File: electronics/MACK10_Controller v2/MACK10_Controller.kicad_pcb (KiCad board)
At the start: 2 copper layers, 57.6 x 67.3 mm, 55 parts, among them J2 Motor, J3 J_Expansion, J4 I/O, J5 Sensor IDC, J6 Interface IDC, J7 Fan, J8 E_STOP, J9 24V IN, Q1 SS8550, U1 TMC2208, U2 HX711, U3 XIAO-C6, U4 INA226, U5 PCF8575, U6 MINI360

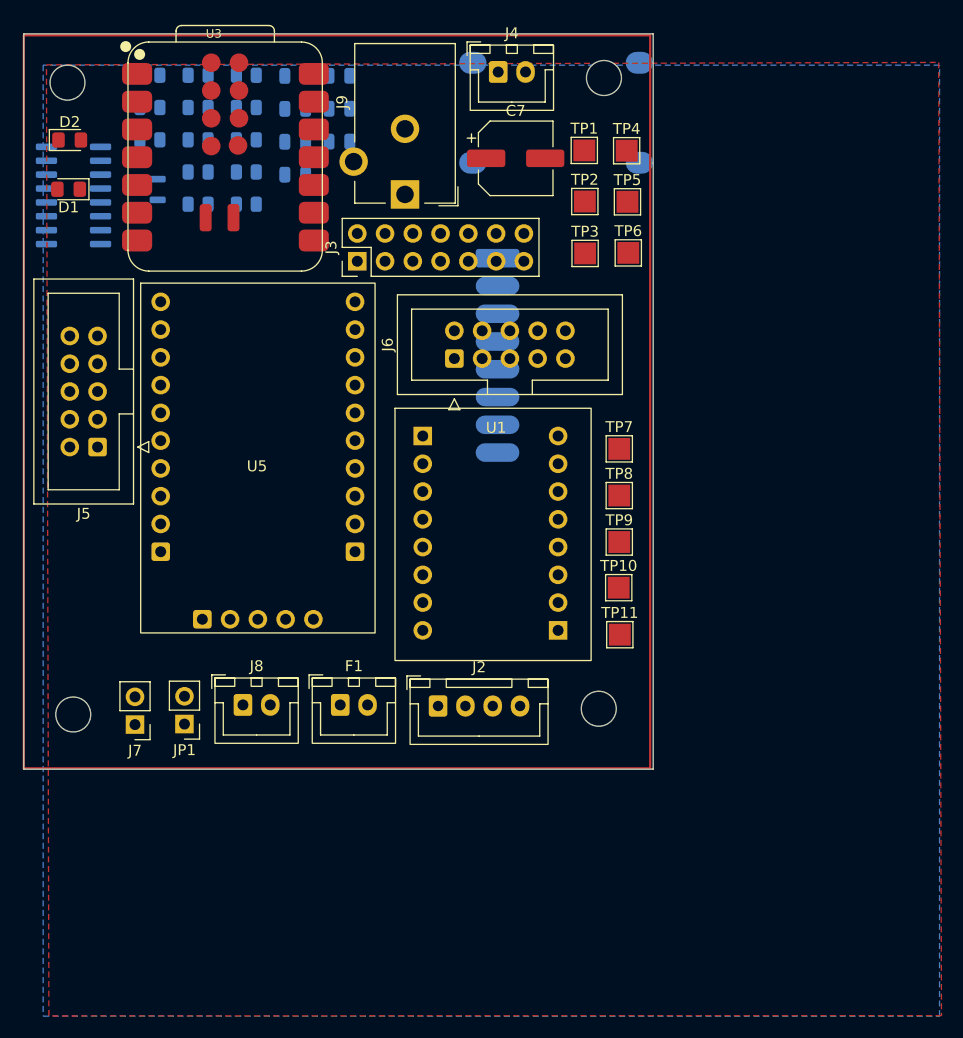
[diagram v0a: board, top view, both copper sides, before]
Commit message: PCB Layout Finalization
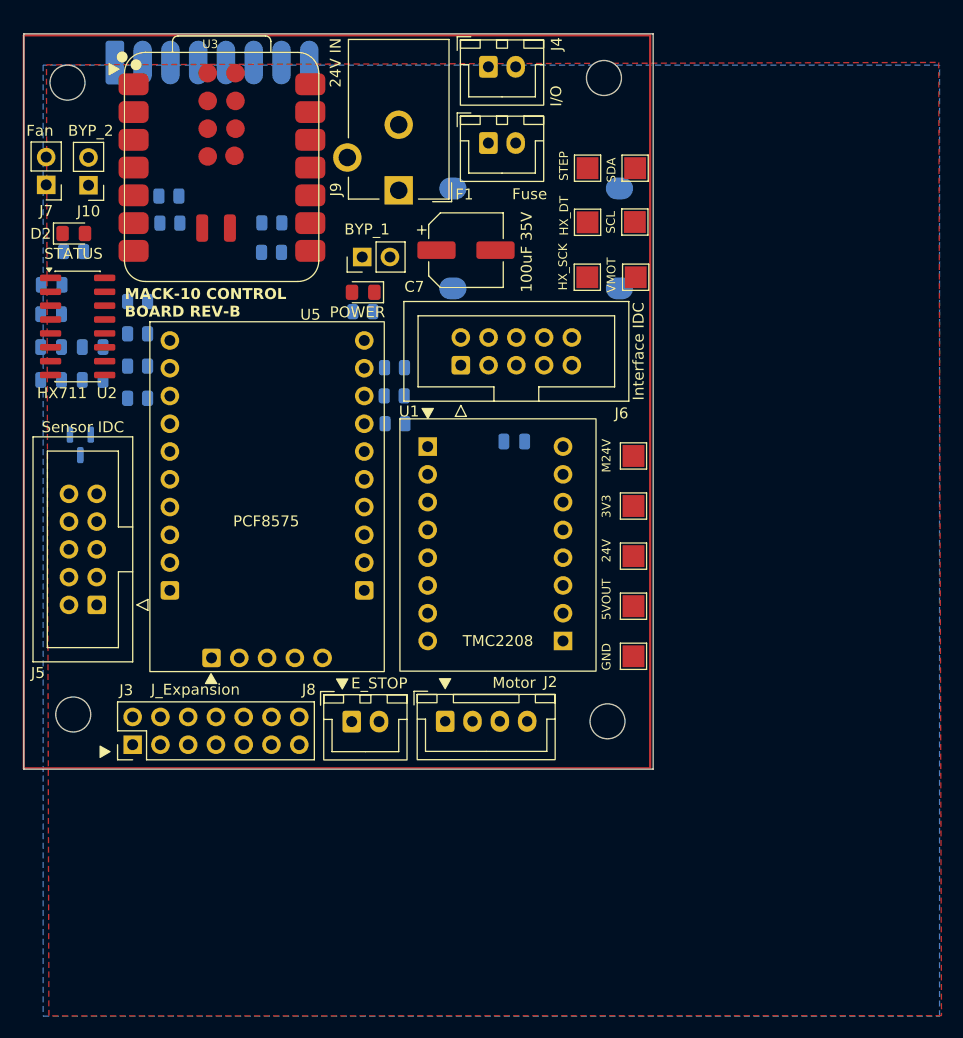
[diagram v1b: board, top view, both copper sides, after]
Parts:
- added J10: BYP_2, Connector_PinHeader_2.54mm:PinHeader_1x02_P2.54mm_Vertical, F.Cu at (23.1, 31.0)
- D2: value SMD_STATUS -> STATUS
- F1: value 2A Fuse -> Fuse
- JP1: value FUSE_BYPASS -> BYP_1
- U2: moved to F.Cu
- moved F1 53.2 mm to (59.7, 27.1)
- moved J7 50.0 mm to (19.3, 30.9)
- moved J3 48.8 mm to (27.2, 82.2)
- moved JP1 45.7 mm to (48.2, 37.5), turned to 90 degrees
- moved C5 37.1 mm to (62.1, 54.4)
- moved R8 31.6 mm to (51.2, 52.8)
- moved C6 31.4 mm to (23.5, 45.8)
- moved C8 31.4 mm to (23.5, 48.8)
- moved C1 29.4 mm to (19.8, 40.1)
- moved C2 29.2 mm to (19.7, 42.8)
- moved C3 29.2 mm to (19.7, 45.8)
- moved C4 29.2 mm to (19.7, 48.8)
- moved D1 28.6 mm to (48.3, 40.8)
- moved R9 27.2 mm to (51.1, 50.2)
- moved R6 26.4 mm to (48.2, 42.5)
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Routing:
- net /GND: track 0.00 -> 1.27 mm
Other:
- board text added: "MACK-10 CONTROL BOARD REV-B"
